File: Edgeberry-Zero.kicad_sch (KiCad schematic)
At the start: 29 parts, among them J1 Molex_KK_1x02_P2.54mm, J2 Raspberry_Pi_2_3, J3 Edgeberry Cartridge Connector, J4 Conn_01x04_Socket, P1 12Vin, Q1 BC547, Q2 BC547, Q3 BC547, SW1 SW_PUSH, U1 24LC256, U2 LM2596S-5.0

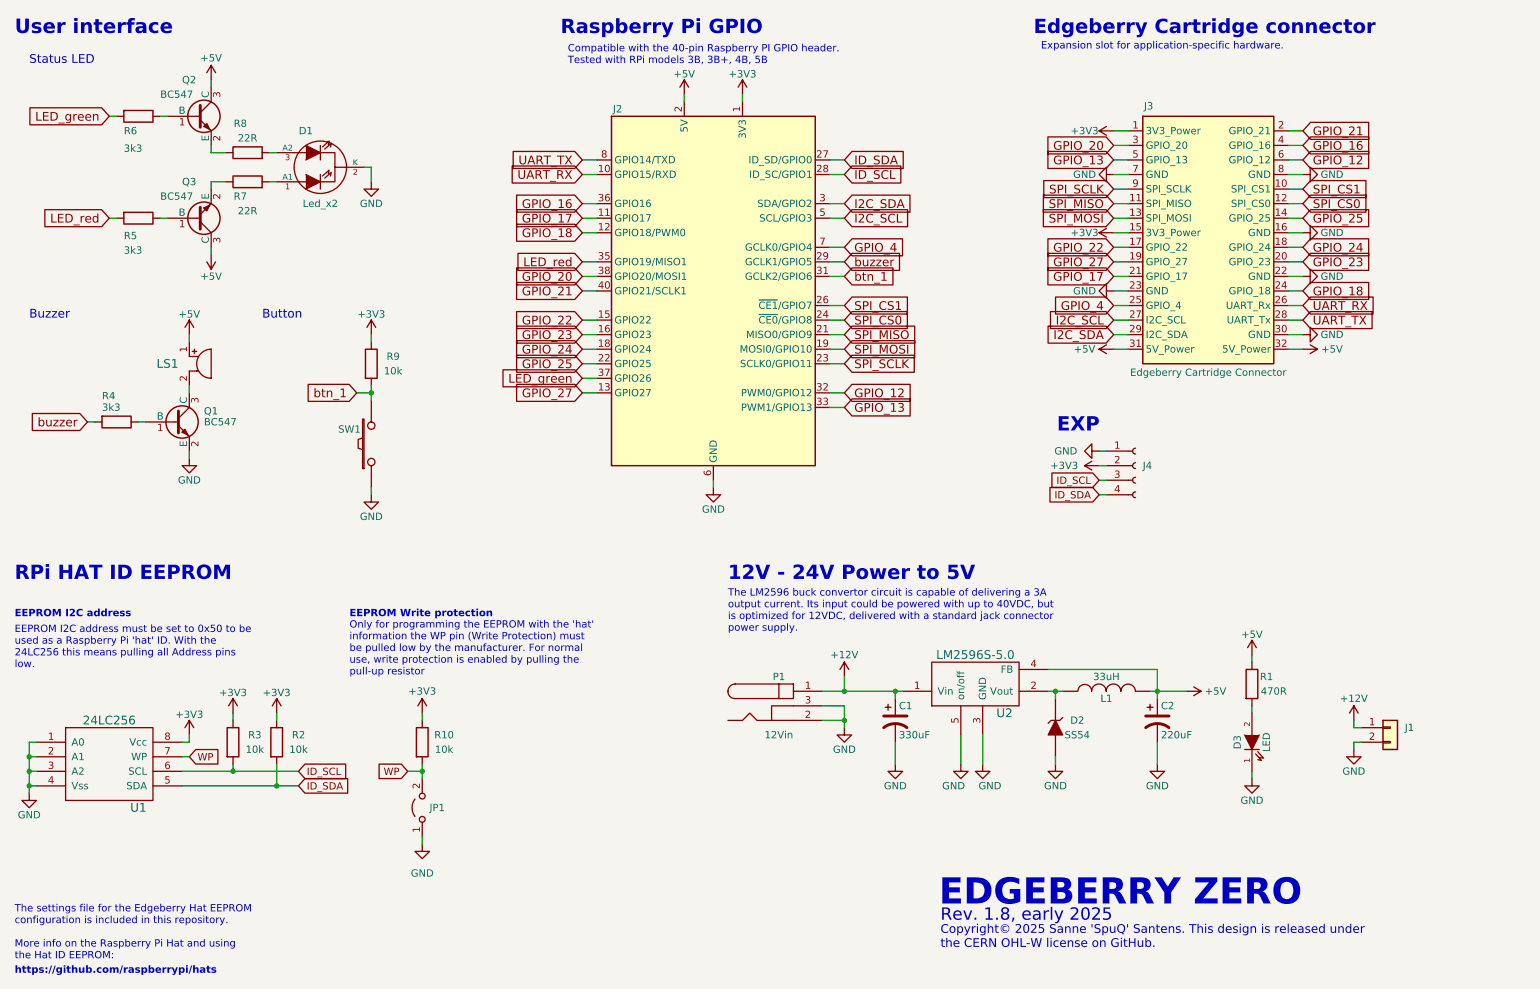
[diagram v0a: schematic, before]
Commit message: Rev 1.8
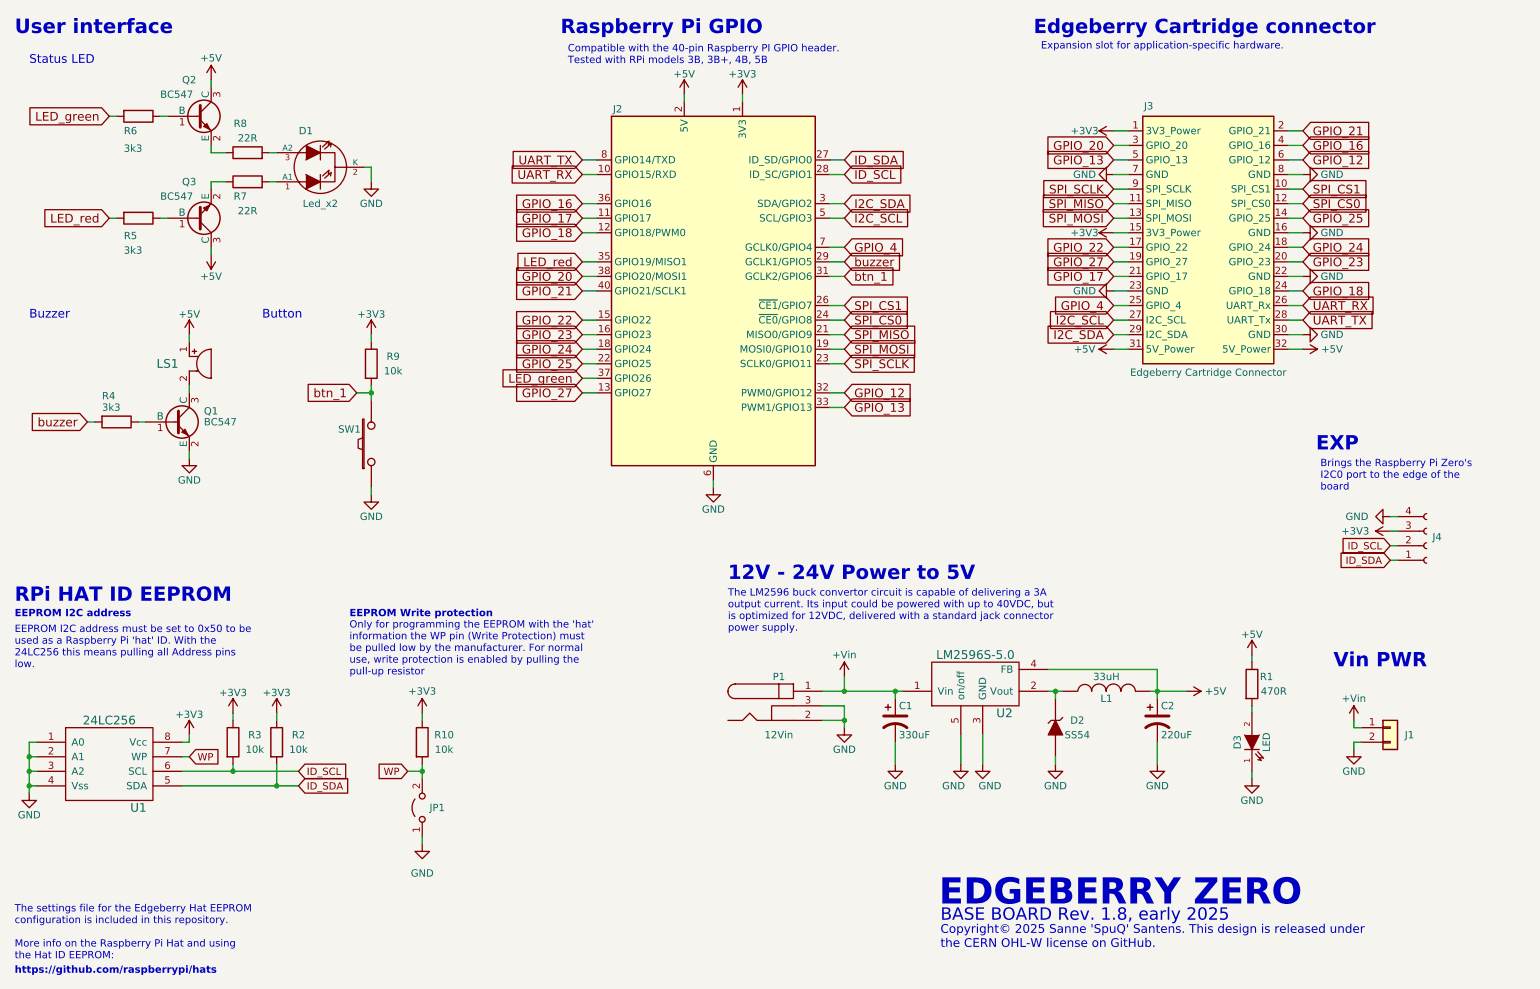
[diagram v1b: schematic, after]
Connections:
- net +3V3: now also J4.3 (Pin_3); no longer J4.2 (Pin_2)
- net GND: now also J4.4 (Pin_4); no longer J4.1 (Pin_1)
- net ID_SCL: now also J4.2 (Pin_2); no longer J4.3 (Pin_3)
- net ID_SDA: now also J4.1 (Pin_1); no longer J4.4 (Pin_4)
- net +12V renamed +Vin
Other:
- note added: "BASE BOARD Rev. 1.8, early 2025"
- note added: "Brings the Raspberry Pi Zero's I2C0 port to the edge of the board"
- note added: "Vin PWR"
- note removed: "Rev. 1.8, early 2025"
- moved on the sheet: J4
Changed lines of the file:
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@@
 		(title "Edgeberry Zero")
 		(date "2024-05-15")
-		(rev "1.7")
+		(rev "1.8")
 	)
 	(junction
@@
 	(wire
 		(pts
-			(xy 209.55 96.52) (xy 210.82 96.52)
+			(xy 260.35 107.95) (xy 261.62 107.95)
 		)
 		(stroke
@@
 	(wire
 		(pts
-			(xy 209.55 99.06) (xy 210.82 99.06)
+			(xy 260.35 110.49) (xy 261.62 110.49)
 		)
 		(stroke
@@
 	(wire
 		(pts
-			(xy 209.55 101.6) (xy 210.82 101.6)
+			(xy 260.35 113.03) (xy 261.62 113.03)
 		)
 		(stroke
@@
 	(wire
 		(pts
-			(xy 209.55 93.98) (xy 210.82 93.98)
+			(xy 260.35 105.41) (xy 261.62 105.41)
 		)
 		(stroke
@@
 		)
 	)
-	(text "Rev. 1.8, early 2025"
+	(text "BASE BOARD Rev. 1.8, early 2025"
 		(exclude_from_sim no)
 		(at 181.864 175.006 0)
@@
 		)
 	)
+	(text "Vin PWR"
+		(exclude_from_sim no)
+		(at 250.444 132.08 0)
+		(effects
+			(font
+				(size 2.4892 2.4892)
+				(thickness 0.4978)
+				(bold yes)
+			)
+			(justify left bottom)
+		)
+	)
+	(text "Brings the Raspberry Pi Zero's\nI2C0 port to the edge of the \nboard"
+		(exclude_from_sim no)
+		(at 248.158 101.092 0)
+		(effects
+			(font
+				(size 1.27 1.27)
+			)
+			(justify left bottom)
+		)
+	)
 	(text "RPi HAT ID EEPROM"
 		(exclude_from_sim no)
-		(at 20.32 116.84 0)
+		(at 20.32 120.65 0)
 		(effects
 			(font
@@
 	(text "EXP"
 		(exclude_from_sim no)
-		(at 202.184 90.932 0)
+		(at 247.396 94.234 0)
 		(effects
 			(font
@@
 	(global_label "ID_SDA"
 		(shape input)
-		(at 209.55 101.6 180)
+		(at 260.35 113.03 180)
 		(fields_autoplaced yes)
 		(effects
@@
 		)
 		(property "Intersheetrefs" "${INTERSHEET_REFS}"
-			(at 200.8085 101.6 0)
+			(at 251.6085 113.03 0)
 			(effects
 				(font
@@
 	(global_label "ID_SCL"
 		(shape input)
-		(at 209.55 99.06 180)
+		(at 260.35 110.49 180)
 		(fields_autoplaced yes)
 		(effects
@@
 		)
 		(property "Intersheetrefs" "${INTERSHEET_REFS}"
-			(at 200.869 99.06 0)
+			(at 251.669 110.49 0)
 			(effects
 				(font
@@
 			)
 		)
-		(property "Value" "+12V"
+		(property "Value" "+Vin"
 			(at 165.1 129.54 0)
 			(effects
@@
 			)
 		)
-		(property "Value" "+12V"
+		(property "Value" "+Vin"
 			(at 254 137.16 0)
 			(effects
@@
 	(symbol
 		(lib_id "EdgeBerry-rescue:+3V3")
-		(at 209.55 96.52 90)
+		(at 260.35 107.95 90)
 		(mirror x)
 		(unit 1)
@@
 		(dnp no)
 		(property "Reference" "#PWR23"
-			(at 213.36 96.52 0)
+			(at 264.16 107.95 0)
 			(effects
 				(font
@@
 		)
 		(property "Value" "+3V3"
-			(at 203.454 96.52 90)
+			(at 254.254 107.95 90)
 			(effects
 				(font
@@
 		)
 		(property "Footprint" ""
-			(at 209.55 96.52 0)
+			(at 260.35 107.95 0)
 			(effects
 				(font
@@
 		)
 		(property "Datasheet" ""
-			(at 209.55 96.52 0)
+			(at 260.35 107.95 0)
 			(effects
 				(font
@@
 		)
 		(property "Description" ""
-			(at 209.55 96.52 0)
+			(at 260.35 107.95 0)
 			(effects
 				(font
@@
 	(symbol
 		(lib_id "power:GND")
-		(at 209.55 93.98 270)
+		(at 260.35 105.41 270)
 		(mirror x)
 		(unit 1)
@@
 		(fields_autoplaced yes)
 		(property "Reference" "#PWR15"
-			(at 203.2 93.98 0)
+			(at 254 105.41 0)
 			(effects
 				(font
@@
 		)
 		(property "Value" "GND"
-			(at 205.74 93.9799 90)
+			(at 256.54 105.4099 90)
 			(effects
 				(font
@@
 		)
 		(property "Footprint" ""
-			(at 209.55 93.98 0)
+			(at 260.35 105.41 0)
 			(effects
 				(font
@@
 		)
 		(property "Datasheet" ""
-			(at 209.55 93.98 0)
+			(at 260.35 105.41 0)
 			(effects
 				(font
@@
 		)
 		(property "Description" ""
-			(at 209.55 93.98 0)
+			(at 260.35 105.41 0)
 			(effects
 				(font
@@
 		(dnp no)
 		(property "Reference" "J1"
-			(at 262.89 142.2399 0)
+			(at 262.89 143.51 0)
 			(effects
 				(font
@@
 	(symbol
 		(lib_id "Connector:Conn_01x04_Socket")
-		(at 215.9 96.52 0)
+		(at 266.7 110.49 0)
+		(mirror x)
 		(unit 1)
 		(exclude_from_sim no)
@@
 		(on_board yes)
 		(dnp no)
-		(fields_autoplaced yes)
 		(property "Reference" "J4"
-			(at 217.17 96.5199 0)
+			(at 267.716 108.966 0)
 			(effects
 				(font
@@
 		)
 		(property "Value" "Conn_01x04_Socket"
-			(at 217.17 99.0599 0)
+			(at 267.97 107.9501 0)
 			(effects
 				(font
@@
 		)
 		(property "Footprint" "Connector_PinSocket_2.00mm:PinSocket_1x04_P2.00mm_Horizontal"
-			(at 215.9 96.52 0)
+			(at 266.7 110.49 0)
 			(effects
 				(font
@@
 		)
 		(property "Datasheet" "~"
-			(at 215.9 96.52 0)
+			(at 266.7 110.49 0)
 			(effects
 				(font
@@
 		)
 		(property "Description" "Generic connector, single row, 01x04, script generated"
-			(at 215.9 96.52 0)
+			(at 266.7 110.49 0)
 			(effects
 				(font
